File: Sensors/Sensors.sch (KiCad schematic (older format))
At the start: 11 parts, among them J1 Conn_01x05, J2 Conn_01x04, J3 Conn_01x02, U1 LIS2DE12, U2 MS5607-02BA

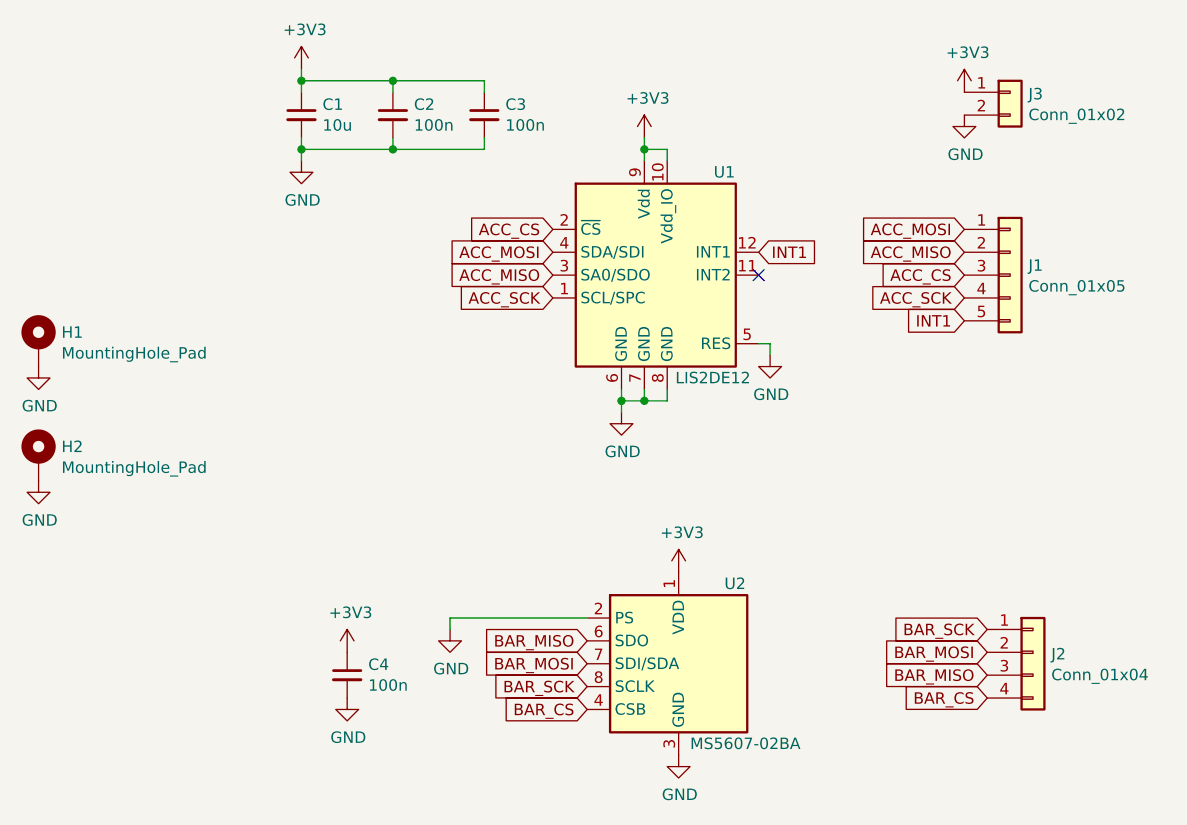
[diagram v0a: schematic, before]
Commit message: Add files via upload
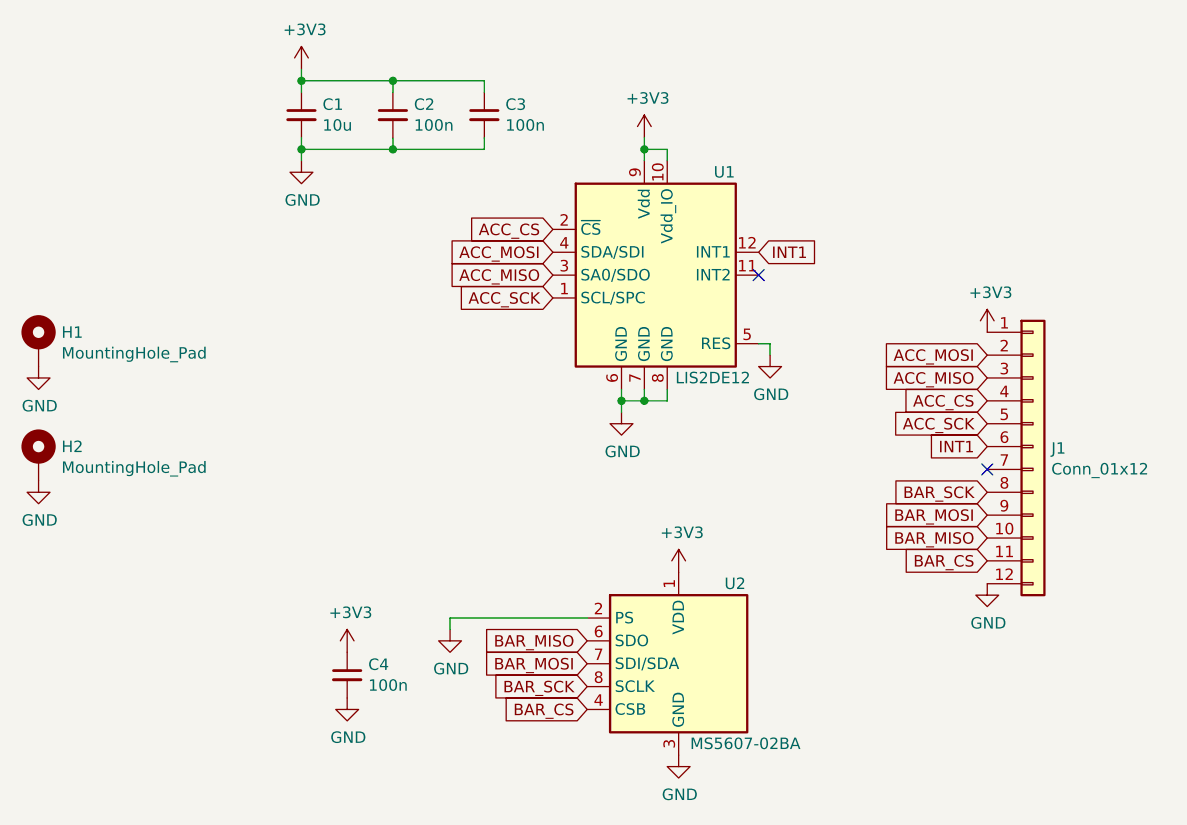
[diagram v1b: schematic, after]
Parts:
- removed J1: Conn_01x05, Connector_PinHeader_2.54mm:PinHeader_1x05_P2.54mm_Vertical, symbol Connector_Generic:Conn_01x05
- removed J2: Conn_01x04, Connector_PinHeader_2.54mm:PinHeader_1x04_P2.54mm_Vertical, symbol Connector_Generic:Conn_01x04
- removed J3: Conn_01x02, Connector_PinHeader_2.54mm:PinHeader_1x02_P2.54mm_Vertical, symbol Connector_Generic:Conn_01x02
- added J1: Conn_01x12, Connector_PinHeader_2.54mm:PinHeader_1x12_P2.54mm_Vertical, symbol Connector_Generic:Conn_01x12
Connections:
- net +3V3: now also J1.1 (Pin_1)
- net ACC_CS: now also J1.4 (Pin_4)
- net ACC_MISO: now also J1.3 (Pin_3)
- net ACC_MOSI: now also J1.2 (Pin_2)
- net ACC_SCK: now also J1.5 (Pin_5)
- net BAR_CS: now also J1.11 (Pin_11)
- net BAR_MISO: now also J1.10 (Pin_10)
- net BAR_MOSI: now also J1.9 (Pin_9)
- net BAR_SCK: now also J1.8 (Pin_8)
- net GND: now also J1.12 (Pin_12)
- net INT1: now also J1.6 (Pin_6)
- no-connect marks 1 -> 2
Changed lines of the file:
@@
 Text GLabel 5600 3500 0    50   Input ~ 0
 ACC_SCK
-Text GLabel 7400 3400 0    50   Input ~ 0
+Text GLabel 7500 3950 0    50   Input ~ 0
 ACC_CS
-Text GLabel 7400 3200 0    50   Input ~ 0
+Text GLabel 7500 3750 0    50   Input ~ 0
 ACC_MOSI
-Text GLabel 7400 3300 0    50   Input ~ 0
+Text GLabel 7500 3850 0    50   Input ~ 0
 ACC_MISO
-Text GLabel 7400 3500 0    50   Input ~ 0
+Text GLabel 7500 4050 0    50   Input ~ 0
 ACC_SCK
-Text GLabel 7400 3600 0    50   Input ~ 0
+Text GLabel 7500 4150 0    50   Input ~ 0
 INT1
 $Comp
@@
 $EndComp
 $Comp
-L Connector_Generic:Conn_01x02 J3
-U 1 1 621490E9
-P 7600 2600
-F 0 "J3" H 7680 2592 50  0000 L CNN
-F 1 "Conn_01x02" H 7680 2501 50  0000 L CNN
-F 2 "Connector_PinHeader_2.54mm:PinHeader_1x02_P2.54mm_Vertical" H 7600 2600 50  0001 C CNN
-F 3 "~" H 7600 2600 50  0001 C CNN
-	1    7600 2600
-	1    0    0    -1
-$EndComp
-$Comp
 L power:+3V3 #PWR0111
 U 1 1 6214A184
-P 7400 2600
-F 0 "#PWR0111" H 7400 2450 50  0001 C CNN
-F 1 "+3V3" H 7415 2773 50  0000 C CNN
-F 2 "" H 7400 2600 50  0001 C CNN
-F 3 "" H 7400 2600 50  0001 C CNN
-	1    7400 2600
+P 7500 3650
+F 0 "#PWR0111" H 7500 3500 50  0001 C CNN
+F 1 "+3V3" H 7515 3823 50  0000 C CNN
+F 2 "" H 7500 3650 50  0001 C CNN
+F 3 "" H 7500 3650 50  0001 C CNN
+	1    7500 3650
 	1    0    0    -1
 $EndComp
@@
 L power:GND #PWR0112
 U 1 1 6214A8B1
-P 7400 2700
-F 0 "#PWR0112" H 7400 2450 50  0001 C CNN
-F 1 "GND" H 7405 2527 50  0000 C CNN
-F 2 "" H 7400 2700 50  0001 C CNN
-F 3 "" H 7400 2700 50  0001 C CNN
-	1    7400 2700
+P 7500 4750
+F 0 "#PWR0112" H 7500 4500 50  0001 C CNN
+F 1 "GND" H 7505 4577 50  0000 C CNN
+F 2 "" H 7500 4750 50  0001 C CNN
+F 3 "" H 7500 4750 50  0001 C CNN
+	1    7500 4750
 	1    0    0    -1
 $EndComp
-$Comp
-L Connector_Generic:Conn_01x04 J2
-U 1 1 6214B921
-P 7700 5050
-F 0 "J2" H 7780 5042 50  0000 L CNN
-F 1 "Conn_01x04" H 7780 4951 50  0000 L CNN
-F 2 "Connector_PinHeader_2.54mm:PinHeader_1x04_P2.54mm_Vertical" H 7700 5050 50  0001 C CNN
-F 3 "~" H 7700 5050 50  0001 C CNN
-	1    7700 5050
-	1    0    0    -1
-$EndComp
-$Comp
-L Connector_Generic:Conn_01x05 J1
-U 1 1 6214C97C
-P 7600 3400
-F 0 "J1" H 7680 3442 50  0000 L CNN
-F 1 "Conn_01x05" H 7680 3351 50  0000 L CNN
-F 2 "Connector_PinHeader_2.54mm:PinHeader_1x05_P2.54mm_Vertical" H 7600 3400 50  0001 C CNN
-F 3 "~" H 7600 3400 50  0001 C CNN
-	1    7600 3400
-	1    0    0    -1
-$EndComp
-Text GLabel 7500 5150 0    50   Input ~ 0
+Text GLabel 7500 4550 0    50   Input ~ 0
 BAR_MISO
-Text GLabel 7500 5050 0    50   Input ~ 0
+Text GLabel 7500 4450 0    50   Input ~ 0
 BAR_MOSI
-Text GLabel 7500 4950 0    50   Input ~ 0
+Text GLabel 7500 4350 0    50   Input ~ 0
 BAR_SCK
-Text GLabel 7500 5250 0    50   Input ~ 0
+Text GLabel 7500 4650 0    50   Input ~ 0
 BAR_CS
 Wire Wire Line
@@
 	1    0    0    -1
 $EndComp
+$Comp
+L Connector_Generic:Conn_01x12 J1
+U 1 1 621C38AD
+P 7700 4150
+F 0 "J1" H 7780 4142 50  0000 L CNN
+F 1 "Conn_01x12" H 7780 4051 50  0000 L CNN
+F 2 "Connector_PinHeader_2.54mm:PinHeader_1x12_P2.54mm_Vertical" H 7700 4150 50  0001 C CNN
+F 3 "~" H 7700 4150 50  0001 C CNN
+	1    7700 4150
+	1    0    0    -1
+$EndComp
+NoConn ~ 7500 4250
 $EndSCHEMATC
